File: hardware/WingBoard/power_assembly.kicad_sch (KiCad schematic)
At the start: 16 parts, among them J201 PWR_SEL, J202 Vin, SW201 SW_POWER, SW202 SW_DPDT_x2, U201 AZ1117-5.0, U202 AZ1117-3.3

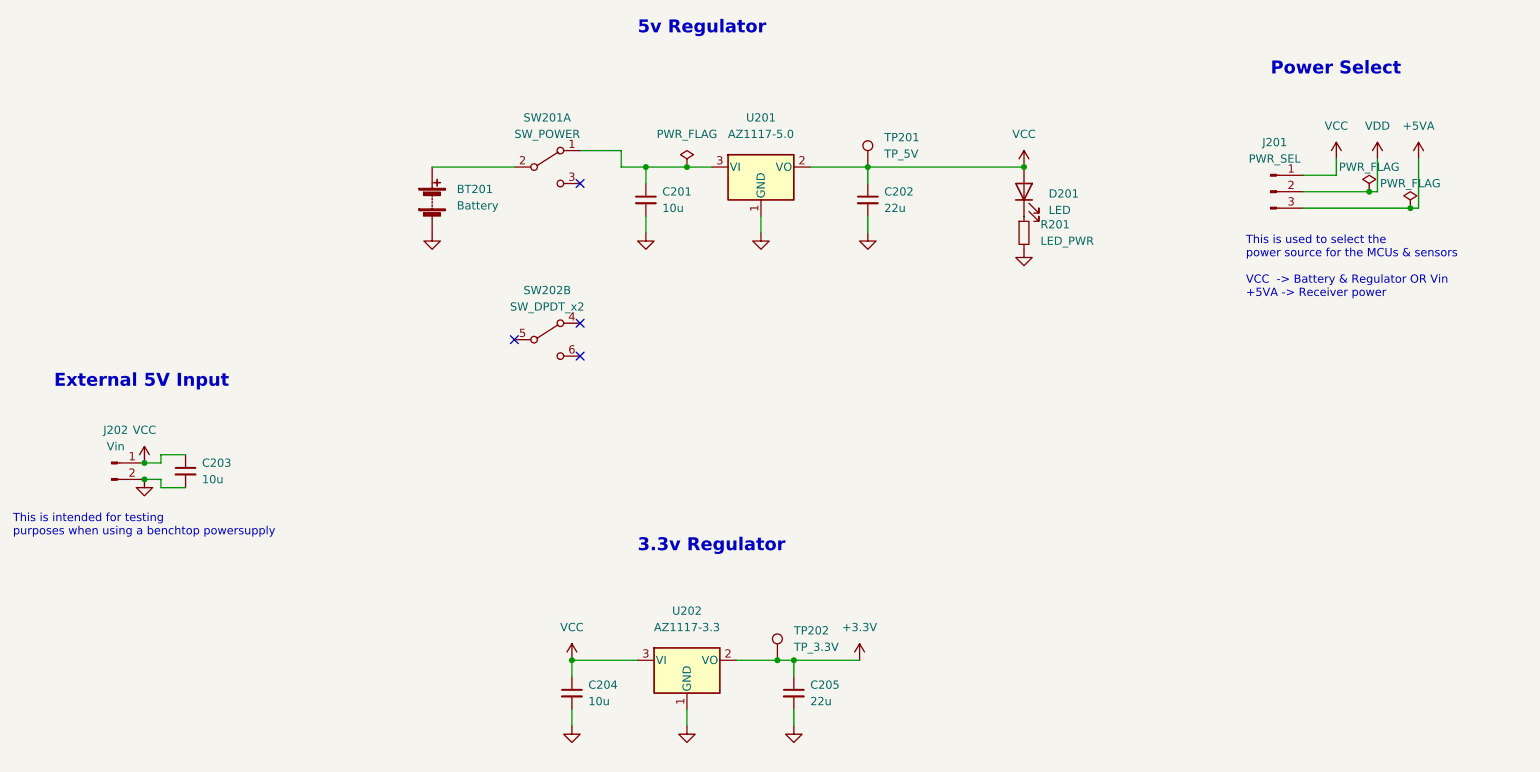
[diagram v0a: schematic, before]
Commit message: Minor hardware design updates and assigned PCB footprints
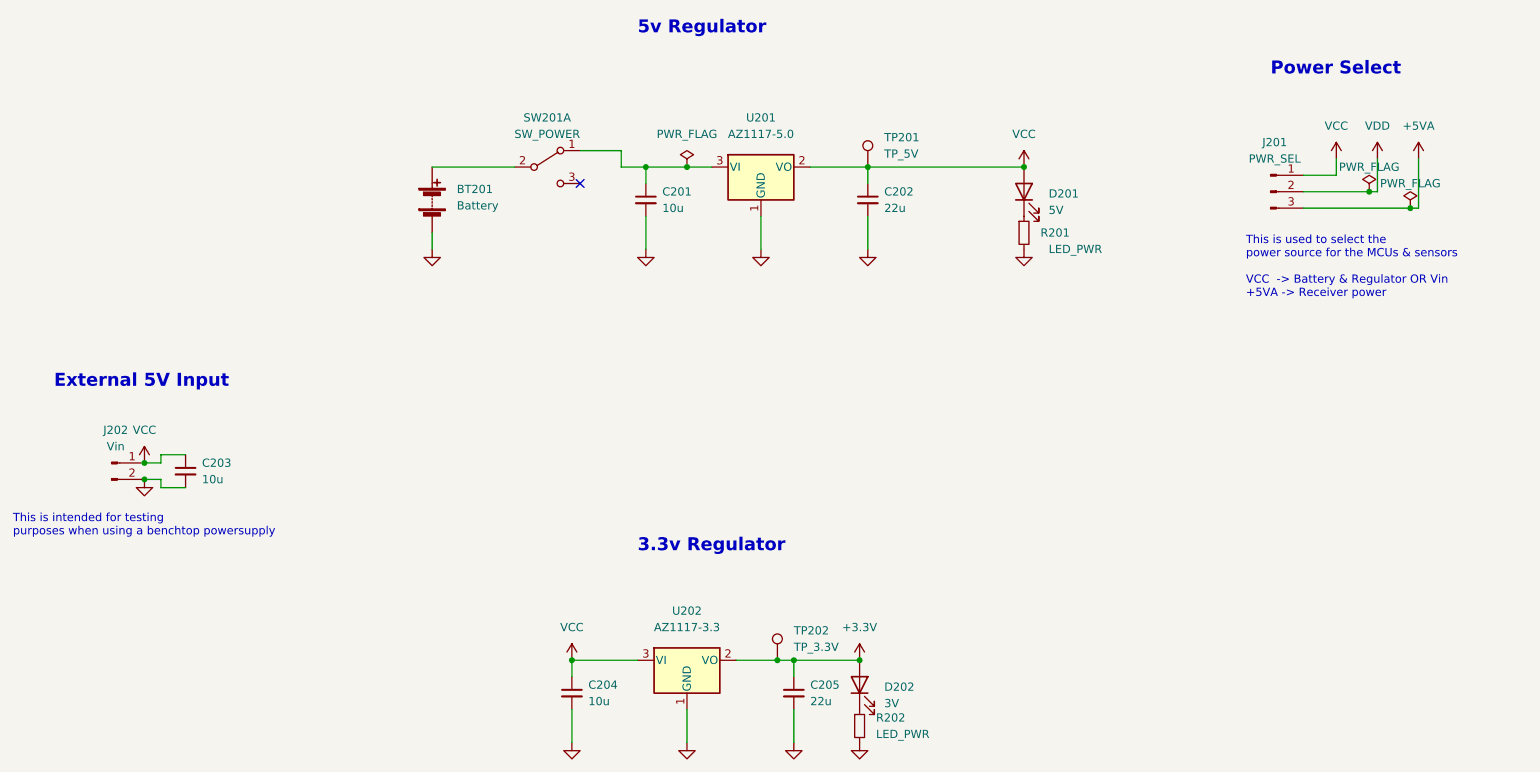
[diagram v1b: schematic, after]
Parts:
- removed SW202: SW_DPDT_x2, symbol Switch:SW_DPDT_x2
- added D202: 3V, LED_SMD:LED_0805_2012Metric_Pad1.15x1.40mm_HandSolder, symbol Device:LED
- added R202: LED_PWR, Resistor_SMD:R_0805_2012Metric_Pad1.20x1.40mm_HandSolder, symbol Device:R_Small
- BT201: footprint (none) -> Connector_AMASS:AMASS_XT30U-M_1x02_P5.0mm_Vertical
- C201, C202, C203, C204, C205: footprint (none) -> Capacitor_SMD:C_0805_2012Metric_Pad1.18x1.45mm_HandSolder
- D201: value LED -> 5V; footprint (none) -> LED_SMD:LED_0805_2012Metric_Pad1.15x1.40mm_HandSolder
- J201: footprint (none) -> Connector_PinHeader_2.54mm:PinHeader_1x03_P2.54mm_Vertical
- J202: footprint (none) -> Connector_PinHeader_2.54mm:PinHeader_1x02_P2.54mm_Vertical
- R201: footprint (none) -> Resistor_SMD:R_0805_2012Metric_Pad1.20x1.40mm_HandSolder
- SW201: footprint (none) -> Button_Switch_SMD:SW_DPDT_MSS22D18_6pin_bje
- TP201, TP202: footprint (none) -> TestPoint:TestPoint_Pad_D1.5mm
- U201: footprint (none) -> ICs:AZ1117CH-5.0TRG1
- U202: footprint (none) -> ICs:AZ1117CR-3.3TRG1
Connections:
- net +3V3: now also D202.2 (A)
- net GND: now also R202.2
- new net: D202.1 (K), R202.1
- no-connect marks 4 -> 1
